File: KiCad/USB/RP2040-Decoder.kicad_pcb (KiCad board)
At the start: 4 copper layers, 30 x 20 mm, 77 parts, among them J1 T0, J10 1, J11 2, J12 3, J13 4, J14 5, J15 +V, J16 M_OUT_B, J17 M_OUT_A, J18 GND, J19 SWCLK, J2 T1, J20 SWDIO, J21 SWDIO, J3 0, J4 1, J5 2, J6 3, J7 +3V3, J8 USB_C_Receptacle_USB2.0, J9 0, Q1 T2N7002BK, Q2 T2N7002BK, Q3 T2N7002BK, Q4 T2N7002BK, Q5 T2N7002BK, SW1 TS-1088-AR02016, U1 AP7381-33Y-13, U2 LM4040C30FTA, U3 DRV8874PWPR, U4 W25Q64JVSSIQ, U5 RP2040, Y1 X322512MSB4SI

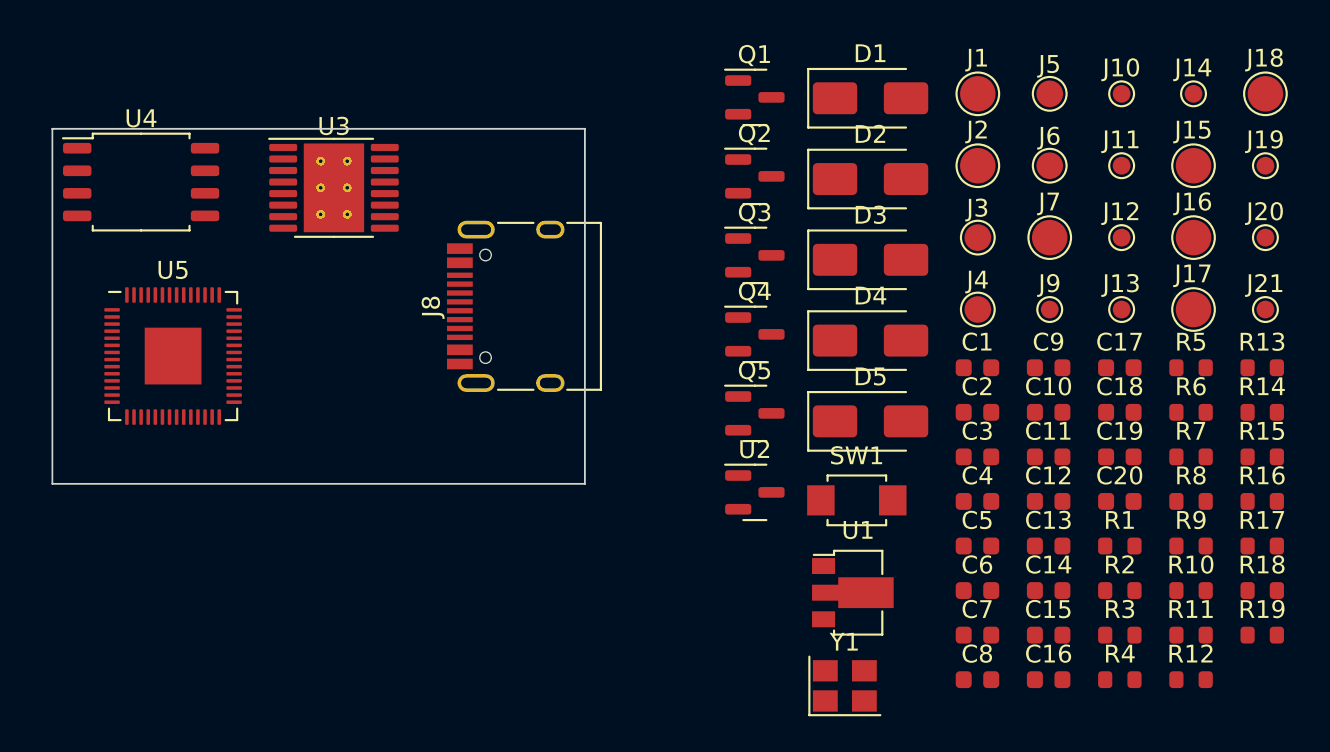
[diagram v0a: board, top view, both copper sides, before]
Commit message: USB PCB routing, minor changes to schematic
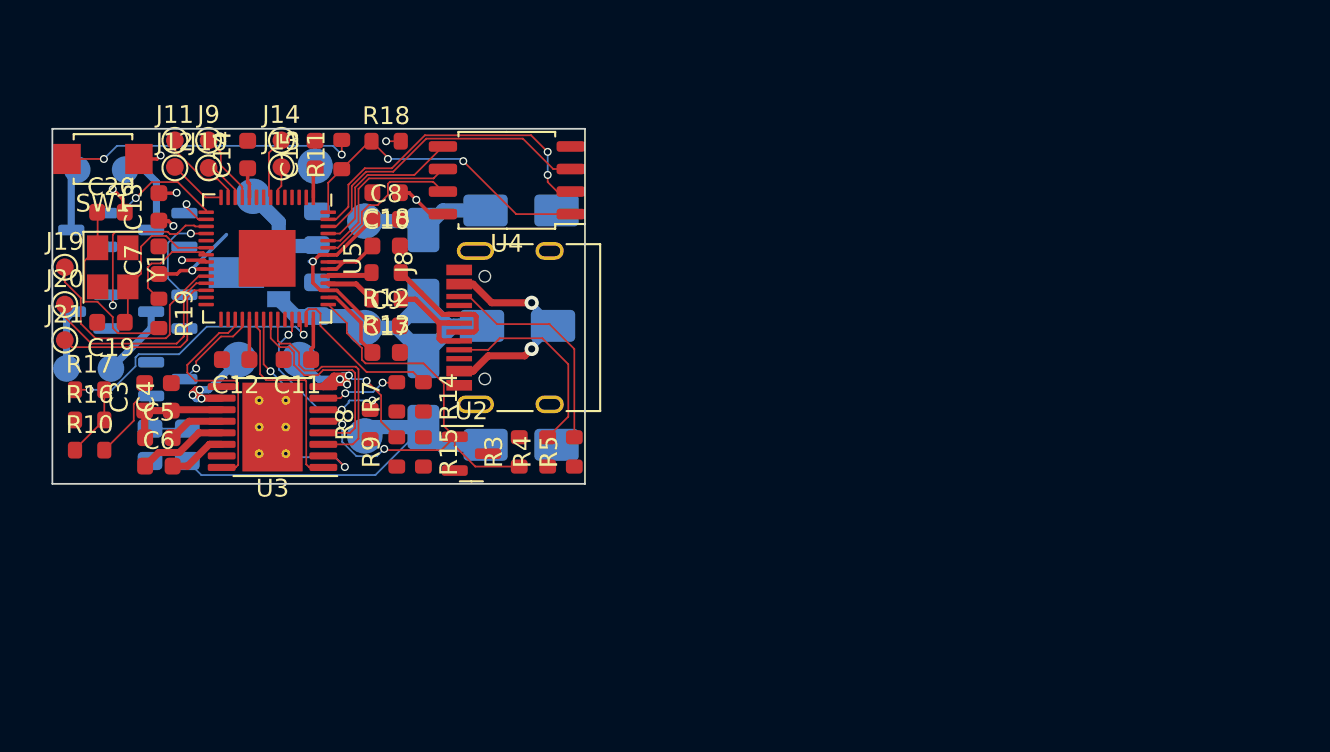
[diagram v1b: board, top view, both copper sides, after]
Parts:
- removed C16: 100n, RP2040-Decoder_Additional_Footprints:C_0603_1608Metric_Removed_Silkscreen
- removed R6: 6k8, RP2040-Decoder_Additional_Footprints:R_0603_1608Metric_Removed_Silkscreen
- C1, C2: footprint RP2040-Decoder_Additional_Footprints:C_0603_1608Metric_Removed_Silkscreen -> Capacitor_SMD:C_0805_2012Metric; moved to B.Cu
- D1, D2, D3, D4, D5, J1, J15, J16, J17, J18, J2, J3, J4, J5, J6, J7, Q1, Q2, Q3, Q4, Q5, U1: moved to B.Cu
- J21: value SWDIO -> RUN
- R1, R2: footprint RP2040-Decoder_Additional_Footprints:R_0603_1608Metric_Removed_Silkscreen -> Resistor_SMD:R_0805_2012Metric; moved to B.Cu
- moved J19 67.9 mm to (20.7, 27.8)
- moved J20 67.7 mm to (20.7, 29.9)
- moved J21 67.7 mm to (20.7, 31.9)
- moved R17 66.6 mm to (22.1, 34.7)
- moved R16 66.2 mm to (22.1, 36.4)
- moved R19 64.7 mm to (26.0, 30.4), turned to -90 degrees
- moved R10 62.5 mm to (22.1, 38.1)
- moved C20 59.1 mm to (23.3, 24.7)
- moved J5 57.5 mm to (20.8, 33.5), turned to 180 degrees
- moved C19 57.3 mm to (23.3, 30.9), turned to 180 degrees
- moved R18 55.5 mm to (38.8, 20.7)
- moved R2 55.2 mm to (25.5, 37.8), turned to 90 degrees
- moved R11 55.0 mm to (36.3, 21.4), turned to 90 degrees
- moved J6 54.1 mm to (23.3, 33.5), turned to 180 degrees
- moved J17 53.9 mm to (30.5, 33.0), turned to 90 degrees
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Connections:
- net Net-(U5-USB_DM) renamed /USB_D_MCU-
- net Net-(U5-USB_DP) renamed /USB_D_MCU+
- Q2 pad 1: /GPIO8 -> /GPIO12
- Q3 pad 1: /GPIO9 -> /GPIO13
- Q4 pad 1: /GPIO10 -> /GPIO14
- Q5 pad 1: /GPIO11 -> /GPIO15
- U3 pad 1: /GPIO23 -> /GPIO22
- U3 pad 16: /GPIO7 -> /GPIO20
- U3 pad 2: /GPIO22 -> /GPIO23
- U3 pad 3: /GPIO6 -> /GPIO25
- U3 pad 4: /GPIO12 -> /GPIO24
- U5 pad 11: /GPIO8 -> Net-(J9-Pin_1)
- U5 pad 12: /GPIO9 -> Net-(J10-Pin_1)
- U5 pad 13: /GPIO10 -> Net-(J11-Pin_1)
- U5 pad 14: /GPIO11 -> Net-(J12-Pin_1)
- U5 pad 15: unconnected-(U5-GPIO12-Pad15) -> /GPIO12
- U5 pad 16: unconnected-(U5-GPIO13-Pad16) -> /GPIO13
- U5 pad 17: unconnected-(U5-GPIO14-Pad17) -> /GPIO14
- U5 pad 18: unconnected-(U5-GPIO15-Pad18) -> /GPIO15
- U5 pad 2: Net-(J9-Pin_1) -> unconnected-(U5-GPIO0-Pad2)
- U5 pad 3: Net-(J10-Pin_1) -> unconnected-(U5-GPIO1-Pad3)
- U5 pad 31: unconnected-(U5-GPIO20-Pad31) -> /GPIO20
- U5 pad 38: /GPIO26 -> unconnected-(U5-GPIO26_ADC0-Pad38)
- U5 pad 4: Net-(J11-Pin_1) -> unconnected-(U5-GPIO2-Pad4)
- U5 pad 40: /ADC_EMF_A -> /ADC_EMF_B
- U5 pad 41: /ADC_EMF_B -> /ADC_EMF_A
- U5 pad 5: Net-(J12-Pin_1) -> unconnected-(U5-GPIO3-Pad5)
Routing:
- net +3V3: track 0.00 -> 28.2 mm, vias 0 -> 4
- net /VREF: track 0.00 -> 26.2 mm, vias 0 -> 2
- net +V: track 0.00 -> 24.1 mm
- net Net-(D1-K): track 0.00 -> 22.2 mm
- net Net-(U4-DO(IO1)): track 0.00 -> 18.7 mm, vias 0 -> 2
- net Net-(U4-~{CS}): track 0.00 -> 18.0 mm, vias 0 -> 2
- net Net-(U4-IO2): track 0.00 -> 17.2 mm
- net Net-(R11-Pad2): track 0.00 -> 16.8 mm, vias 0 -> 2
- net /ADC_EMF_B: track 0.00 -> 15.8 mm, vias 0 -> 2
- net +1V1: track 0.00 -> 15.7 mm, vias 0 -> 2
- net Net-(J19-Pin_1): track 0.00 -> 13.4 mm
- net /GPIO20: track 0.00 -> 13.1 mm
- net /GPIO25: track 0.00 -> 13.0 mm
- net /MOTOR_OUT_A: track 0.00 -> 13.0 mm, vias 0 -> 4
- net /GPIO23: track 0.00 -> 12.9 mm, vias 0 -> 2
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
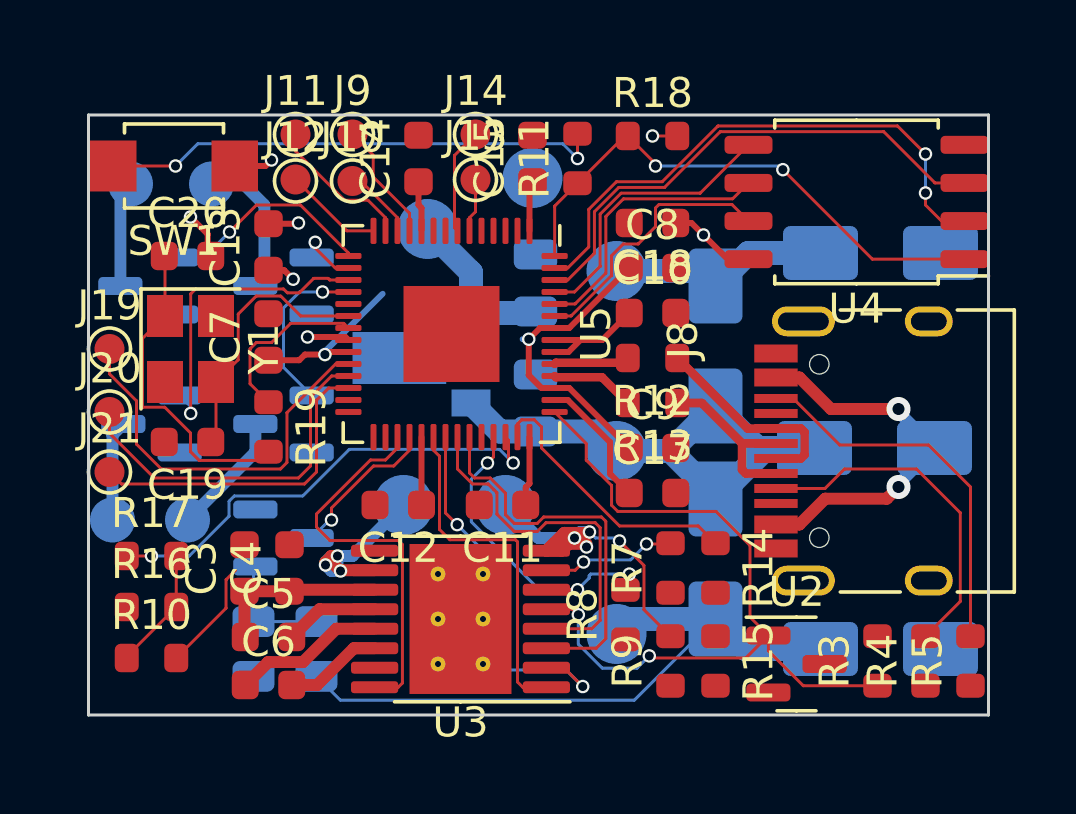
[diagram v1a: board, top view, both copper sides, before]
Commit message: PCB Routing
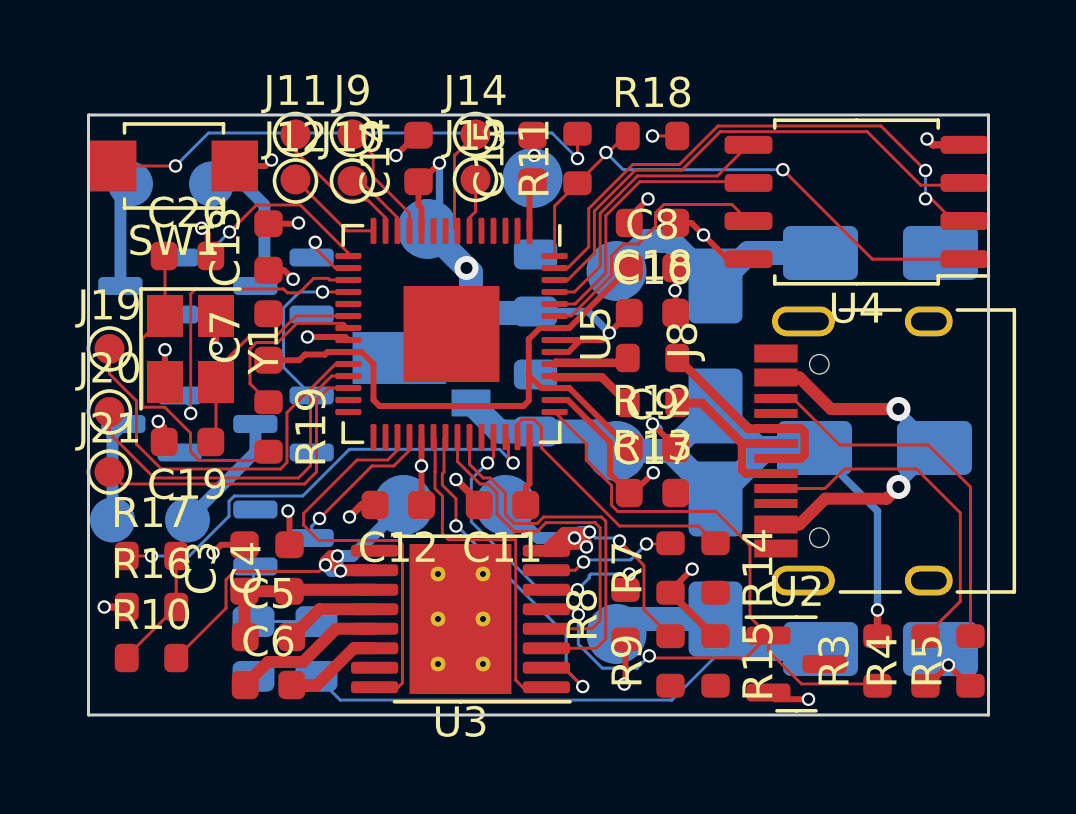
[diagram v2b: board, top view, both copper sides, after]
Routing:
- net GND: track 3.46 -> 26.4 mm, vias 3 -> 21
- net +3V3: track 28.2 -> 35.3 mm, vias 4 -> 9
- net +V: track 24.1 -> 31.3 mm, vias 0 -> 1
- net +1V1: track 15.7 -> 21.0 mm, vias 2 -> 0
- net /MOTOR_OUT_B: track 10.7 -> 13.8 mm
- net Net-(U5-XIN): track 8.84 -> 7.63 mm
- net /GPIO23: track 12.9 -> 11.8 mm
- net /GPIO20: track 13.1 -> 14.0 mm
- net Net-(D3-K): track 7.46 -> 8.29 mm
- net Net-(D1-K): track 22.2 -> 22.9 mm
- net /GPIO24: track 12.8 -> 12.1 mm
- net Net-(U4-~{CS}): track 18.0 -> 18.7 mm
- added copper zone on In2.Cu, net +3V3
- added copper zone on In1.Cu, net GND

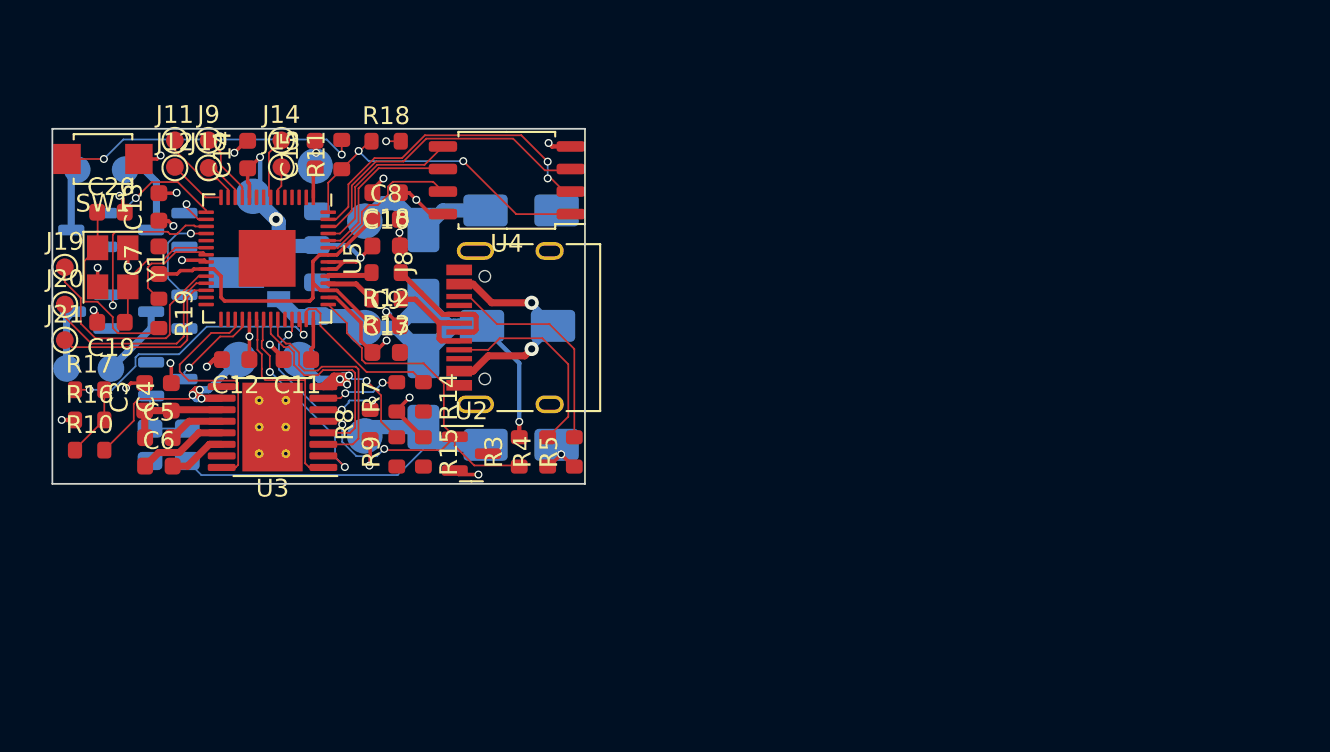
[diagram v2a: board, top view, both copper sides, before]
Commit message: PCB routing
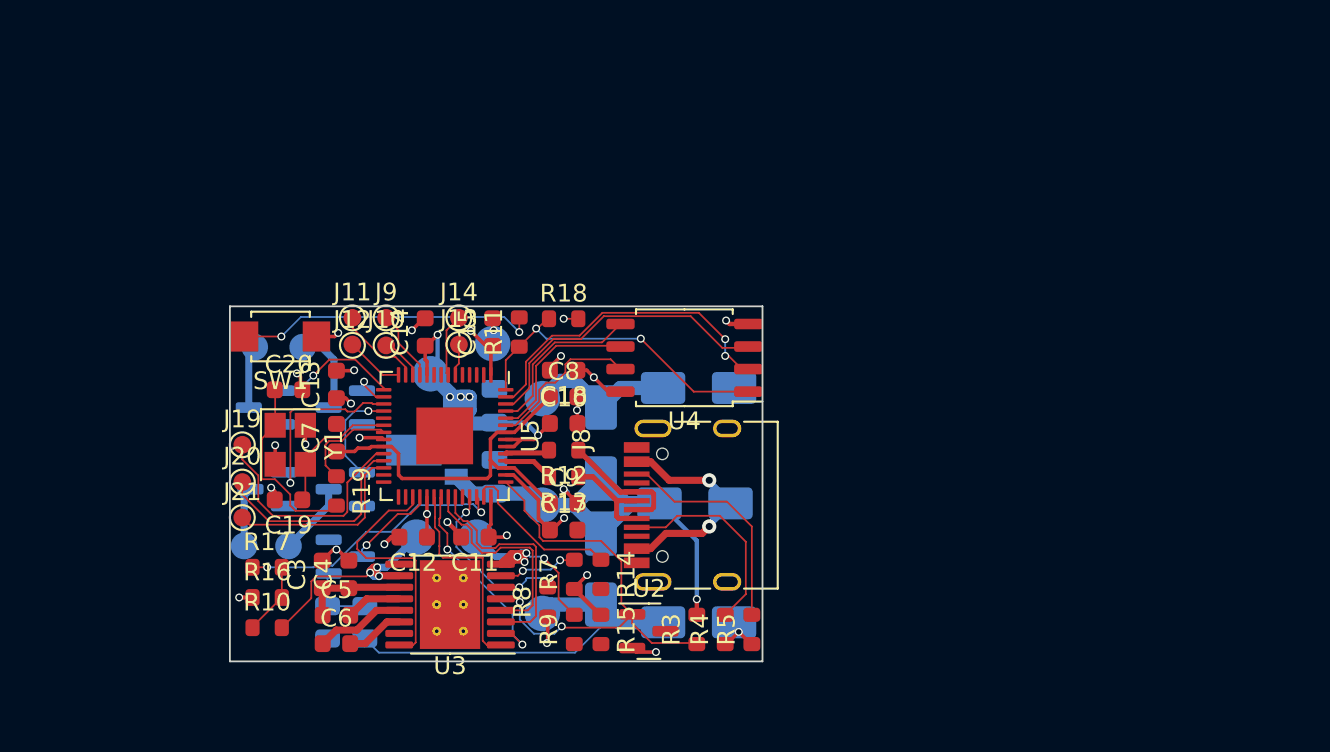
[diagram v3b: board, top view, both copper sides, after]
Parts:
- moved C12 14.1 mm to (40.3, 43.0)
- moved C3 14.1 mm to (35.2, 45.1)
- moved C4 14.1 mm to (36.7, 45.1)
- moved D4 14.1 mm to (50.9, 37.7)
- moved J12 14.1 mm to (36.9, 32.2)
- moved J15 14.1 mm to (47.6, 41.2)
- moved J2 14.1 mm to (47.6, 35.2)
- moved J8 14.1 mm to (57.0, 41.2)
- moved Q2 14.1 mm to (32.0, 35.7)
- moved Q3 14.1 mm to (36.5, 35.7)
- moved C1 14.1 mm to (44.9, 39.6)
- moved C10 14.1 mm to (48.8, 36.6)
- moved C11 14.1 mm to (43.8, 43.0)
- moved C13 14.1 mm to (36.0, 34.4)
- moved C14 14.1 mm to (41.0, 31.4)
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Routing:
- net +3V3: track 35.3 -> 43.9 mm, vias 9 -> 13
- net GND: track 26.4 -> 26.1 mm, vias 21 -> 20
